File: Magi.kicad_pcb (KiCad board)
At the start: 6 copper layers, 122 x 84 mm, 366 parts, among them J1 Micro_SD_Card_Det2, J10 USB_C_Receptacle_USB2.0_16P, J11 USB_C_Receptacle_USB2.0_16P, J2 Bus_M.2_Socket_M, J3 Micro_SD_Card_Det2, J4 Bus_M.2_Socket_M, J5 Micro_SD_Card_Det2, J6 Bus_M.2_Socket_M, J7 RJ45_LED_Shielded, J8 Debug, J9 Magi Connector, Q1 DMN32D2LFB4, Q10 DMN32D2LFB4, Q11 DMN32D2LFB4, Q12 DMN32D2LFB4, Q13 DMN32D2LFB4, Q2 DMN32D2LFB4, Q3 DMN32D2LFB4, Q4 DMN32D2LFB4, Q5 DMN32D2LFB4, Q9 DMN32D2LFB4, T1 GA021G00, T2 GA021G00, T3 GA021G00, T4 GA021G00, U1 RT9742GGJ5, U10 DS1307Z+, U11 TPS56339DDC, U12 TPS56339DDC, U13 RTL8367N, U14 TPD4EUSB30, U15 TPD4EUSB30, U16 TPS259474A, U17 W25Q128JVS, U18 RP2040, U19 TVS2200DRV, U2 DS1307Z+, U20 ESD122DMYR, U21 ESD122DMYR, U22 TPD4EUSB30, U23 TPD4EUSB30, U24 TVS2200DRV, U25 TPS259470A, U26 TPS259474A, U27 TPS62933, U28 TPS259470A, U29 CYPD3177-24LQ, U3 TPS56339DDC, U30 TPS62933, U31 74LVC1G07, U32 74LVC1G07, U33 74LVC1G07, U4 TPS56339DDC, U5 RT9742GGJ5, U6 DS1307Z+, U7 TPS56339DDC, U8 TPS56339DDC, U9 RT9742GGJ5, Y1 32.768kHz, Y2 32.768kHz, Y3 32.768kHz, Y4 25MHz, Y5 ABM8-272-T3

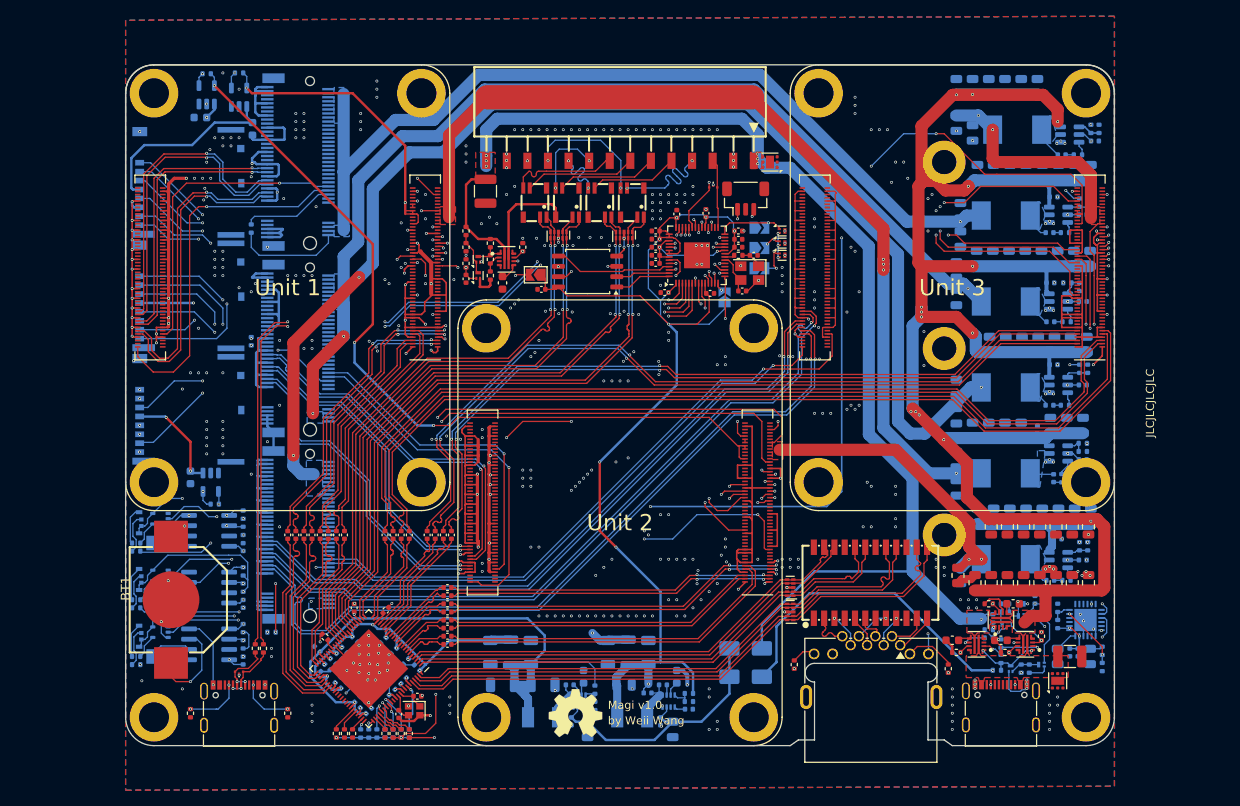
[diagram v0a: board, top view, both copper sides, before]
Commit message: Magi v2.0
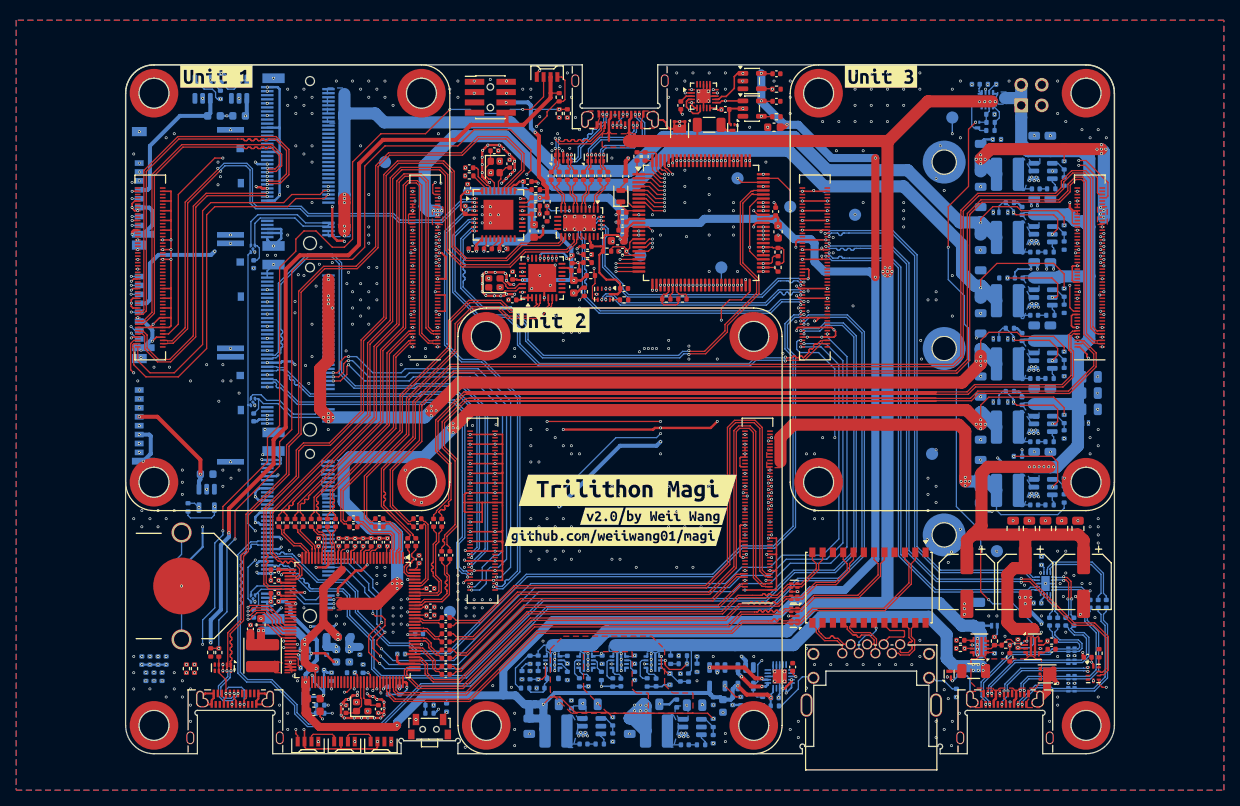
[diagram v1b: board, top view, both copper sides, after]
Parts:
- removed the C10 at (114.5, 109.5)
- removed the C11 at (204.5, 95.1)
- removed the C12 at (206.5, 95.1)
- removed the C13 at (208.5, 95.1)
- removed the C132 at (175.6, 72.5)
- removed the C137 at (164.4, 127.5)
- removed the C143 at (219.0, 123.0)
- removed the C2 at (120.0, 108.0)
- removed the C22 at (207.1, 63.3)
- removed the C68 at (135.0, 108.0)
- removed JP1, JP2, JP3: Unit PWR JP, Jumper:SolderJumper-2_P1.3mm_Open_TrianglePad1.0x1.5mm
- removed JP4: PWR JP, Jumper:SolderJumper-2_P1.3mm_Open_TrianglePad1.0x1.5mm
- removed JP5: POE JP, Jumper:SolderJumper-2_P1.3mm_Open_TrianglePad1.0x1.5mm
- removed Q10, Q11, Q12, Q13, Q5, Q9: DMN32D2LFB4, Package_DFN_QFN:Diodes_DFN1006-3
- removed the R1 at (101.3, 109.0)
- removed the R2 at (114.0, 51.0)
- removed the R3 at (114.5, 107.5)
- removed the R4 at (114.5, 105.5)
- removed the R69 at (211.5, 124.5)
- removed the R8 at (115.5, 70.2)
- removed SYM1: Magi v1.0, Magi:NAMEPLATE
- removed T1, T2, T3, T4: GA021G00, Magi:FILTER-SMD_6P-L4.5-W3.4_GA021G00
- removed the U1 at (114.0, 54.0)
- removed the U2 at (110.3, 107.5)
- removed Y5: ABM8-272-T3, Crystal:Crystal_SMD_3225-4Pin_3.2x2.5mm
- added C135: 6.8n, Capacitor_SMD:C_0402_1005Metric, B.Cu at (157.1, 126.2)
- added C144: 22u, Capacitor_SMD:C_0805_2012Metric, B.Cu at (170.2, 129.0)
- added C153: 22u, Capacitor_SMD:C_0805_2012Metric, F.Cu at (213.5, 107.2)
- added C185: 100n, Capacitor_SMD:C_0402_1005Metric, F.Cu at (156.5, 63.7)
- added C186: 100n, Capacitor_SMD:C_0402_1005Metric, F.Cu at (152.5, 63.7)
- added C187: 100n, Capacitor_SMD:C_0402_1005Metric, F.Cu at (153.5, 63.7)
- added C188: 100n, Capacitor_SMD:C_0402_1005Metric, F.Cu at (154.5, 63.7)
- added C189: 100n, Capacitor_SMD:C_0402_1005Metric, F.Cu at (155.5, 63.7)
- added C25: 100n, Capacitor_SMD:C_0402_1005Metric, B.Cu at (210.6, 83.6)
- added C26: 22u, Capacitor_SMD:C_0805_2012Metric, B.Cu at (212.1, 98.7)
- added C27: 22u, Capacitor_SMD:C_0805_2012Metric, B.Cu at (214.1, 98.7)
- added C28: 100n, Capacitor_SMD:C_0402_1005Metric, B.Cu at (210.2, 99.7)
- added C29: 100n, Capacitor_SMD:C_0402_1005Metric, B.Cu at (212.1, 88.7)
- added C30: 22u, Capacitor_SMD:C_0805_2012Metric, B.Cu at (205.5, 84.1)
- added C92: 100n, Capacitor_SMD:C_0402_1005Metric, B.Cu at (122.5, 127.5)
- added D10: WS2812B, Magi:LED-SMD_4P-L4.0-W1.7-R, F.Cu at (131.5, 133.5)
- added D11: 4.3v, Diode_SMD:D_SOD-523, B.Cu at (167.2, 125.8)
- added D12: 4.3v, Diode_SMD:D_SOD-523, B.Cu at (152.7, 125.7)
- added D13: RB161QS, Diode_SMD:D_SOD-882, B.Cu at (218.4, 94.2)
- added D14: RB161QS, Diode_SMD:D_SOD-882, B.Cu at (207.2, 119.2)
- added D15: RB161QS, Diode_SMD:D_SOD-882, B.Cu at (202.8, 125.0)
- added D6: RB161QS, Diode_SMD:D_SOD-882, B.Cu at (209.2, 91.6)
- added D7: WS2812B, Magi:LED-SMD_4P-L4.0-W1.7-R, F.Cu at (152.0, 51.5)
- added D8: WS2812B, Magi:LED-SMD_4P-L4.0-W1.7-R, F.Cu at (122.5, 133.5)
- added D9: WS2812B, Magi:LED-SMD_4P-L4.0-W1.7-R, F.Cu at (127.0, 133.5)
- added J12: USB_C_Receptacle, Magi:USB-C-SMD_TYPE-C-GT-USB-7007C, F.Cu at (161.0, 54.7)
- added L9: 5.6uH, Inductor_SMD:L_Changjiang_FTC404030S, B.Cu at (165.5, 132.2)
- added R10: 5.1k, Resistor_SMD:R_0402_1005Metric, F.Cu at (163.1, 61.3)
- added R100: 30R, Resistor_SMD:R_0402_1005Metric, B.Cu at (171.0, 133.9)
- added R101: 12k, Resistor_SMD:R_0402_1005Metric, B.Cu at (172.5, 133.2)
- added R102: 5.1k, Resistor_SMD:R_0402_1005Metric, B.Cu at (148.9, 125.3)
- added R103: 5.1k, Resistor_SMD:R_0402_1005Metric, B.Cu at (213.0, 111.2)
- added R104: 5.1k, Resistor_SMD:R_0402_1005Metric, B.Cu at (175.9, 128.5)
- added R105: 5.1k, Resistor_SMD:R_0402_1005Metric, B.Cu at (178.6, 128.5)
- added R106: 5.1k, Resistor_SMD:R_0402_1005Metric, F.Cu at (157.4, 76.0)
- added R107: 5.1k, Resistor_SMD:R_0402_1005Metric, F.Cu at (152.0, 68.8)
- added R108: 5.1k, Resistor_SMD:R_0402_1005Metric, F.Cu at (152.0, 66.9)
- added R109: 5.1k, Resistor_SMD:R_0402_1005Metric, F.Cu at (157.0, 74.4)
- added R11: 5.1k, Resistor_SMD:R_0402_1005Metric, F.Cu at (164.1, 61.3)
- added R110: 5.1k, Resistor_SMD:R_0402_1005Metric, F.Cu at (157.0, 73.4)
- added R111: 5.1k, Resistor_SMD:R_0402_1005Metric, F.Cu at (180.3, 53.0)
- added R112: 5.1k, Resistor_SMD:R_0402_1005Metric, F.Cu at (180.3, 56.4)
- added R113: 5.1k, Resistor_SMD:R_0402_1005Metric, B.Cu at (139.6, 129.3)
- added R114: 5.1k, Resistor_SMD:R_0402_1005Metric, F.Cu at (220.1, 122.6)
- added R115: 5.1k, Resistor_SMD:R_0402_1005Metric, F.Cu at (161.5, 79.0)
- added R5: 5.1k, Resistor_SMD:R_0402_1005Metric, B.Cu at (208.3, 76.3)
- added R66: 1.3k, Resistor_SMD:R_0402_1005Metric, F.Cu at (208.6, 121.6)
- added R7: 5.1k, Resistor_SMD:R_0402_1005Metric, B.Cu at (209.1, 67.0)
- added R74: 1k, Resistor_SMD:R_0402_1005Metric, B.Cu at (160.1, 126.2)
- added R9: 12k, Resistor_SMD:R_0402_1005Metric, B.Cu at (111.7, 53.7)
- added R92: 1.3k, Resistor_SMD:R_0402_1005Metric, B.Cu at (206.7, 57.1)
- added R93: 12k, Resistor_SMD:R_0402_1005Metric, B.Cu at (160.1, 133.0)
- added R94: 5.6k, Resistor_SMD:R_0402_1005Metric, B.Cu at (206.7, 56.1)
- added R95: 5.1k, Resistor_SMD:R_0402_1005Metric, B.Cu at (170.5, 124.4)
- added R97: 64.9k, Resistor_SMD:R_0402_1005Metric, B.Cu at (172.5, 131.2)
- added R98: 1.2k 0.5W, Resistor_SMD:R_1206_3216Metric, F.Cu at (172.0, 57.4)
- added R99: 100k, Resistor_SMD:R_0402_1005Metric, B.Cu at (149.9, 123.4)
- added SW1: SW_Push, Magi:SW-SMD_L4.7-W3.5-P3.35-EH, F.Cu at (137.5, 131.7)
- added TP1: TestPoint, TestPoint:TestPoint_Pad_D1.5mm, B.Cu at (190.0, 68.5)
- added TP10: TestPoint, TestPoint:TestPoint_Pad_D1.5mm, B.Cu at (218.9, 76.0)
- added TP11: TestPoint, TestPoint:TestPoint_Pad_D1.5mm, B.Cu at (207.5, 110.0)
- added TP12: TestPoint, TestPoint:TestPoint_Pad_D1.5mm, B.Cu at (132.0, 62.0)
- added TP13: TestPoint, TestPoint:TestPoint_Pad_D1.5mm, B.Cu at (140.0, 117.5)
- added TP2: TestPoint, TestPoint:TestPoint_Pad_D1.5mm, B.Cu at (199.5, 98.0)
- added TP3: TestPoint, TestPoint:TestPoint_Pad_D1.5mm, B.Cu at (202.0, 56.5)
- added TP4: TestPoint, TestPoint:TestPoint_Pad_D1.5mm, B.Cu at (163.5, 73.5)
- added TP5: TestPoint, TestPoint:TestPoint_Pad_D1.5mm, B.Cu at (175.5, 64.0)
- added TP6: TestPoint, TestPoint:TestPoint_Pad_D1.5mm, B.Cu at (182.0, 67.5)
- added TP7: TestPoint, TestPoint:TestPoint_Pad_D1.5mm, B.Cu at (173.5, 75.0)
- added TP8: TestPoint, TestPoint:TestPoint_Pad_D1.5mm, B.Cu at (175.2, 121.6)
- added TP9: TestPoint, TestPoint:TestPoint_Pad_D1.5mm, B.Cu at (158.2, 121.0)
- added U3: AP2151W, Package_TO_SOT_SMD:SOT-23-5, B.Cu at (109.5, 53.0)
- added U34: TPD4EUSB30, Package_SON:USON-10_2.5x1.0mm_P0.5mm, B.Cu at (216.7, 122.9)
- added U35: AP2151W, Package_TO_SOT_SMD:SOT-23-5, B.Cu at (173.0, 125.5)
- added U36: AP2151W, Package_TO_SOT_SMD:SOT-23-5, B.Cu at (176.5, 125.5)
- added U37: TS3USB221, Package_DFN_QFN:Texas_UQFN-10_1.5x2mm_P0.5mm, F.Cu at (159.0, 78.3)
- added U38: TPD6S300A, Package_DFN_QFN:WQFN-20-1EP_3x3mm_P0.4mm_EP1.7x1.7mm_ThermalVias, F.Cu at (171.3, 53.9)
- added U39: TVS2200DRV, Package_SON:WSON-6-1EP_2x2mm_P0.65mm_EP1x1.6mm, F.Cu at (168.3, 57.9)
- added U4: 74AUP1G125, Package_SON:Texas_X2SON-5_0.8x0.8mm_P0.48mm, B.Cu at (115.7, 72.7)
- added U40: HD3SS460, Magi:WQFN-28-1EP_3.5x5.5mm_P0.5mm_EP2.05x4.05mm_ThermalVias_SingleSided, F.Cu at (156.0, 69.5)
- added U41: TPD4EUSB30, Package_SON:USON-10_2.5x1.0mm_P0.5mm, F.Cu at (158.0, 61.5)
- added U42: AP2151W, Package_TO_SOT_SMD:SOT-23-5, F.Cu at (177.3, 52.0)
- added U43: TPD4EUSB30, Package_SON:USON-10_2.5x1.0mm_P0.5mm, F.Cu at (154.0, 61.5)
- added U44: AP2151W, Package_TO_SOT_SMD:SOT-23-5, F.Cu at (177.3, 55.4)
- added kibuzzard-69C4E3CF: G***, kibuzzard-69C4E3CF, B.Cu at (115.6, 69.0)
- added kibuzzard-69C4E40D: G***, kibuzzard-69C4E40D, B.Cu at (115.6, 83.0)
- added kibuzzard-69C4E42D: G***, kibuzzard-69C4E42D, B.Cu at (115.6, 97.0)
- added kibuzzard-69C50949: G***, kibuzzard-69C50949, F.Cu at (111.2, 51.4)
- added kibuzzard-69C5095C: G***, kibuzzard-69C5095C, F.Cu at (152.5, 81.5)
- added kibuzzard-69C50974: G***, kibuzzard-69C50974, F.Cu at (193.2, 51.4)
- added kibuzzard-69C50981: G***, kibuzzard-69C50981, B.Cu at (196.5, 52.4)
- added kibuzzard-69C5098A: G***, kibuzzard-69C5098A, B.Cu at (196.5, 75.4)
- added kibuzzard-69C509A0: G***, kibuzzard-69C509A0, B.Cu at (196.5, 98.4)
- added kibuzzard-6A5B14ED: G***, kibuzzard-6A5B14ED, F.Cu at (161.9, 102.5)
- added kibuzzard-6A5B154C: G***, kibuzzard-6A5B154C, F.Cu at (167.7, 105.7)
- added kibuzzard-6A5B1551: G***, kibuzzard-6A5B1551, F.Cu at (160.2, 108.2)
- added kibuzzard-6A5B157A: G***, kibuzzard-6A5B157A, F.Cu at (158.8, 105.7)
- BT1: value RTC Battery -> CR1220
- C100, C113: value 100u -> 100n; footprint Capacitor_SMD:C_1206_3216Metric -> Capacitor_SMD:C_0402_1005Metric; moved to F.Cu
- C101, C102, C104, C105, C106, C111, C114, C115, C154, C155, C162, C163, C40, C70, C78, C91, C93: moved to F.Cu
- C103, C108: value 100n -> 4.7u; footprint Capacitor_SMD:C_0402_1005Metric -> Capacitor_SMD:C_0603_1608Metric; moved to F.Cu
- C109: value 6p -> 100n
- C110: value 6p -> 4.7u; footprint Capacitor_SMD:C_0402_1005Metric -> Capacitor_SMD:C_0603_1608Metric
- C112, C99: value 100u -> 10u; footprint Capacitor_SMD:C_1206_3216Metric -> Capacitor_SMD:C_0603_1608Metric; moved to F.Cu
- C116: value 100n -> 1u; moved to F.Cu
- C117: value 1u -> 100n
- C118, C96: value 100n -> 1u
- C119, C127, C128: value 100n -> 18pf
- C120: value 1u -> 18pf
- C122: value 6.8n -> 100n; footprint Capacitor_SMD:C_0603_1608Metric -> Capacitor_SMD:C_0402_1005Metric
- C123: value 3.3u 100V -> 100n; footprint Capacitor_SMD:C_1210_3225Metric -> Capacitor_SMD:C_0402_1005Metric
- C124, C125: value 15p -> 100n
- C129, C32, C36, Q1, Q2: moved to B.Cu
- C13: renamed from C9; value 10u 25V -> 10u
- C130, C131: value 100n -> 6.8n; moved to B.Cu
- C132: renamed from C135; footprint Capacitor_SMD:C_0603_1608Metric -> Capacitor_SMD:C_0402_1005Metric
- C133: value 100n -> 10u 50V; footprint Capacitor_SMD:C_0402_1005Metric -> Capacitor_SMD:C_1210_3225Metric; moved to B.Cu
- C134: value 3.3u 100V -> 100n; footprint Capacitor_SMD:C_1210_3225Metric -> Capacitor_SMD:C_0402_1005Metric; moved to B.Cu
- C136: value 100n -> 6.8n
- C137: renamed from C144; footprint Capacitor_SMD:C_0603_1608Metric -> Capacitor_SMD:C_0402_1005Metric
- C138, C148: value 10u 50V -> 22u
- C139: value 100n 50V -> 100n
- C14, C145, C168, C169, C175, C176, C177, C178, C179, C181, C182, C183, C184, C51, C54, C71, C72, C76, C86: value 22u -> 100n; footprint Capacitor_SMD:C_0805_2012Metric -> Capacitor_SMD:C_0402_1005Metric
- C140: value 1u 50V -> 100n; footprint Capacitor_SMD:C_0805_2012Metric -> Capacitor_SMD:C_0402_1005Metric
- C141, C142, C147, C48: value 100n -> 22u; footprint Capacitor_SMD:C_0402_1005Metric -> Capacitor_SMD:C_0805_2012Metric
- C143: renamed from C153; footprint Capacitor_SMD:C_0603_1608Metric -> Capacitor_SMD:C_0402_1005Metric; moved to B.Cu
- C146: value 33n -> 100n; footprint Capacitor_SMD:C_0603_1608Metric -> Capacitor_SMD:C_0402_1005Metric
- C149: value 100n 50V -> 22u; footprint Capacitor_SMD:C_0402_1005Metric -> Capacitor_SMD:C_0805_2012Metric
- C150: value 100u -> 22u; footprint Capacitor_SMD:C_1206_3216Metric -> Capacitor_SMD:C_0805_2012Metric
- C151: value 100u -> 22u; footprint Capacitor_SMD:C_1206_3216Metric -> Capacitor_SMD:C_0805_2012Metric; moved to F.Cu
- C152: value 33n -> 22u; footprint Capacitor_SMD:C_0603_1608Metric -> Capacitor_SMD:C_0805_2012Metric; moved to F.Cu
- C157, C158, C159: value 22u -> 100u; footprint Capacitor_SMD:C_0805_2012Metric -> Capacitor_SMD:CP_Elec_6.3x5.7; moved to F.Cu
- C167: value 1u -> 100n; moved to B.Cu
- C170, C172, C173, C174, C50: value 22u -> 100n; footprint Capacitor_SMD:C_0805_2012Metric -> Capacitor_SMD:C_0402_1005Metric; moved to B.Cu
- C171: value 22u -> 10u; footprint Capacitor_SMD:C_0805_2012Metric -> Capacitor_SMD:C_0603_1608Metric; moved to B.Cu
- C180, C79: value 22u -> 10u; footprint Capacitor_SMD:C_0805_2012Metric -> Capacitor_SMD:C_0603_1608Metric
- C21, C41, C42, C43, C44, C59, C60, C75, C81, C82, C83, C84, C85, C89, C90: value 22u -> 100n; footprint Capacitor_SMD:C_0805_2012Metric -> Capacitor_SMD:C_0402_1005Metric; moved to F.Cu
- C31, C33, C34: value 100n -> 22u; footprint Capacitor_SMD:C_0402_1005Metric -> Capacitor_SMD:C_0805_2012Metric; moved to B.Cu
- C35: value 100n -> 10u; footprint Capacitor_SMD:C_0402_1005Metric -> Capacitor_SMD:C_0603_1608Metric; moved to B.Cu
- C39, C69: value 10u 25V -> 100n; footprint Capacitor_SMD:C_0603_1608Metric -> Capacitor_SMD:C_0402_1005Metric; moved to F.Cu
- C57, C95: value 100n -> 10u; footprint Capacitor_SMD:C_0402_1005Metric -> Capacitor_SMD:C_0603_1608Metric
- C73, C74: value 22u -> 18pf; footprint Capacitor_SMD:C_0805_2012Metric -> Capacitor_SMD:C_0402_1005Metric; moved to F.Cu
- C80: value 22u -> 1u; footprint Capacitor_SMD:C_0805_2012Metric -> Capacitor_SMD:C_0402_1005Metric
- C97, C98: value 100n -> 10u; footprint Capacitor_SMD:C_0402_1005Metric -> Capacitor_SMD:C_0603_1608Metric; moved to F.Cu
- D1, D2, D3: value LED_Dual_AAKK -> RB161QS; footprint Magi:LED-ARRAY-SMD_4P-L3.0-W1.5-L-FD -> Diode_SMD:D_SOD-882
- D4, D5: value M7 -> RB161QS; footprint Diode_SMD:D_SMA -> Diode_SMD:D_SOD-882
- FB1, FB2: value FerriteBead -> 220R; footprint Inductor_SMD:L_1206_3216Metric -> Inductor_SMD:L_0603_1608Metric
- J1, J3, J5: footprint Magi:TF-SMD_503398-1892 -> Magi:SDCARD_MOLEX_503398-1892
- J10: value USB_C_Receptacle_USB2.0_16P -> Conn_02x02_Odd_Even; footprint Magi:USB-C-SMD_TYPEC-304J-BCP16 -> Connector_PinHeader_2.54mm:PinHeader_2x02_P2.54mm_Vertical; moved to B.Cu
- J11: value USB_C_Receptacle_USB2.0_16P -> USB_C_Receptacle; footprint Magi:USB-C-SMD_TYPEC-304J-BCP16 -> Magi:USB-C-SMD_TYPE-C-GT-USB-7007C
- J7: footprint Magi:RJ45-TH_MJ88B-B011-RVL11-P -> Magi:RJ45-TH_RJ45-005-202-11
- J8: value Debug -> USB_C_Receptacle; footprint Connector_JST:JST_SH_BM03B-SRSS-TB_1x03-1MP_P1.00mm_Vertical -> Magi:USB-C-SMD_TYPE-C-GT-USB-7007C
- J9: value Magi Connector -> Conn_02x04; footprint Magi:HDR-SMD_14P-P2.54-H-F-L11.5 -> Magi:PinHeader_2x04_P1.27mm_Vertical_SMD_MountingPegs
- L1, L2: footprint Inductor_SMD:L_Sunlord_MWSA0603S -> Inductor_SMD:L_Changjiang_FTC404030S
- L3, L5: value 5.6uH -> 4.7uH; footprint Inductor_SMD:L_Sunlord_MWSA0603S -> Inductor_SMD:L_Changjiang_FTC404030S
- L4, L6: value 4.7uH -> 5.6uH; footprint Inductor_SMD:L_Sunlord_MWSA0603S -> Inductor_SMD:L_Changjiang_FTC404030S
- L7: value 2.2u 4.5A -> 2.2uH; footprint Inductor_SMD:L_Sunlord_MWSA0402S -> Inductor_SMD:L_Changjiang_FTC404030S; moved to F.Cu
- L8: value 2.2u 4.5A -> 4.7uH; footprint Inductor_SMD:L_Sunlord_MWSA0402S -> Inductor_SMD:L_Changjiang_FTC404030S
- Module1, Module2, Module3: value ComputeModule4-CM4 -> Compute Module
- R1: renamed from R5; value 52.3k 1% -> 64.9k
- R12, R23, R88: value 1k -> 37.4k
- R13, R24: value 12k 1% -> 64.9k
- R14, R15, R25, R26: value 4.7k -> 30R
- R16, R27: value 52.3k 1% -> 5.1k
- R17, R28: value 30 1% -> 12k
- R18, R29: value 10k 1% -> 5.1k
- R19, R30: value 10k -> 12k
- R2: renamed from R9; value 30.9k 1% -> 37.4k
- R20, R31: value 30.9k 1% -> 12k
- R21, R32: value 30 1% -> 5.1k; moved to F.Cu
- R22, R33: value 10k 1% -> 5.1k; moved to F.Cu
- R3: renamed from R6; value 30 1% -> 30R
- R34: value 2.49K -> 5.1k; moved to B.Cu
- R35, R38: value 4.7k -> 5.1k
- R36, R39, R40: value 4.7k -> 5.1k; moved to B.Cu
- R37: value 4.7k -> 2.49K
- R4: renamed from R10; value 30 1% -> 30R
- R41, R42, R43: value 4.7k -> 1k; moved to B.Cu
- R44, R45, R47, R48, R49, R50: value 4.7k -> 1k
- R46: value 470R -> 1k; moved to B.Cu
- R51: value 470R -> 100k
- R52: value 4.7k -> 100k; moved to F.Cu
- R53: value 100k -> 5.1k
- R54: value 220k 1% -> 5.1k
- R55, R82: value 20k -> 5.1k
- R56: value 2.74k 1% -> 12k
- R57: value 12.7k 1% -> 5.1k
- R58: value 27.4 -> 5.1k
- R59: value 27.4 -> 100k
- R6: renamed from R7; value 10k 1% -> 12k
- R60: value 4.7k -> 100k
- R61: value 1k -> 5.1k
- R63: value 5.1k -> 2.49K
- R64: value 220k 1% -> 100k; moved to F.Cu
- R65: value 220k 1% -> 100k; moved to B.Cu
- R67: value 220k 1% -> 5.6k
- R68, R80: value 100k -> 1.3k
- R69: renamed from R66; value 100k -> 12k
- R70: value 2.26k 1% -> 5.1k
- R71: value 953 -> 5.1k; moved to B.Cu
- R72: value 13k 1% -> 5.6k; moved to F.Cu
- R73: value 30.9k 1% -> 100k
- R75, R85: value 10k 1% -> 1k
- R76: value 15k -> 1k; footprint Capacitor_SMD:C_0402_1005Metric -> Resistor_SMD:R_0402_1005Metric; moved to F.Cu
- R77: value 220k 1% -> 100k
- R79: value 2.74k 1% -> 5.6k
- R8: renamed from R11; value 10k 1% -> 12k
- R81: value 2.4k -> 5.1k
- R83: value 12.7k 1% -> 100k
- R84: value 3.74k 1% -> 1k
- R86: renamed from R74; value 953 -> 1k
- R87, R91: value 1k -> 100k
- R89: value 1k -> 30R
- R90: value 5.1k -> 1.2k 0.5W; footprint Resistor_SMD:R_0402_1005Metric -> Resistor_SMD:R_1206_3216Metric; moved to F.Cu
- R96: renamed from R86; value 1.2k 1% -> 1k; moved to B.Cu
- TR1: value H2456G -> H2449G; footprint Magi:XFMR-SMD-24_L16.6-W9.0-LS9.6-BL -> Magi:RJ45-SMD_24P_L15.6-W8.7_H24308C
- U10, U6: value DS1307Z+ -> TPS56339DDC; footprint Package_SO:SOIC-8_3.9x4.9mm_P1.27mm -> Package_TO_SOT_SMD:SOT-23-6
- U11, U7: value TPS56339DDC -> AP2151W; footprint Package_TO_SOT_SMD:SOT-23-6 -> Package_TO_SOT_SMD:SOT-23-5
- U12, U8: value TPS56339DDC -> 74AUP1G125; footprint Package_TO_SOT_SMD:SOT-23-6 -> Package_SON:Texas_X2SON-5_0.8x0.8mm_P0.48mm
- U13: value RTL8367N -> RTL8367S-CG; footprint Magi:QFN-88_EP_10x10_Pitch0.4mm2 -> Package_QFP:LQFP-128_14x14mm_P0.4mm
- U14, U15: footprint Magi:USON-10_2.5x1.0mm_P0.5mm -> Package_SON:USON-10_2.5x1.0mm_P0.5mm
- U16: value TPS259474A -> USB2514B; footprint Magi:RPW0010A-MFG -> Package_DFN_QFN:QFN-36-1EP_6x6mm_P0.5mm_EP3.7x3.7mm
- U17: value W25Q128JVS -> CH390H; footprint Package_SO:SOIC-8_5.23x5.23mm_P1.27mm -> Package_DFN_QFN:QFN-32-1EP_5x5mm_P0.5mm_EP3.45x3.45mm
- U18: value RP2040 -> STM32G0B1VETx; footprint Package_DFN_QFN:QFN-56-1EP_7x7mm_P0.4mm_EP3.2x3.2mm -> Package_QFP:LQFP-100_14x14mm_P0.5mm
- U19: value TVS2200DRV -> TPD4EUSB30; footprint Package_SON:WSON-6-1EP_2x2mm_P0.65mm_EP1x1.6mm -> Package_SON:USON-10_2.5x1.0mm_P0.5mm
- U20, U21: value ESD122DMYR -> TPS259470A; footprint Magi:DMY0003A -> Magi:RPW0010A-MFG; moved to B.Cu
- U22: value TPD4EUSB30 -> TPS259470A; footprint Magi:USON-10_2.5x1.0mm_P0.5mm -> Magi:RPW0010A-MFG
- U23: value TPD4EUSB30 -> TPS259470A; footprint Magi:USON-10_2.5x1.0mm_P0.5mm -> Magi:RPW0010A-MFG; moved to B.Cu
- U24: value TVS2200DRV -> TPS259470A; footprint Package_SON:WSON-6-1EP_2x2mm_P0.65mm_EP1x1.6mm -> Magi:RPW0010A-MFG; moved to B.Cu
- U26: value TPS259474A -> TPS56339DDC; footprint Magi:RPW0010A-MFG -> Package_TO_SOT_SMD:SOT-23-6; moved to B.Cu
- U27: value TPS62933 -> TPS259470A; footprint Package_TO_SOT_SMD:SOT-583-8 -> Magi:RPW0010A-MFG
- U28: value TPS259470A -> TPS56339DDC; footprint Magi:RPW0010A-MFG -> Package_TO_SOT_SMD:SOT-23-6; moved to B.Cu
- U29: value CYPD3177-24LQ -> TVS2200DRV; footprint Package_DFN_QFN:QFN-24-1EP_4x4mm_P0.5mm_EP2.75x2.75mm -> Package_SON:WSON-6-1EP_2x2mm_P0.65mm_EP1x1.6mm; moved to F.Cu
- U30: value TPS62933 -> TPD6S300A; footprint Package_TO_SOT_SMD:SOT-583-8 -> Package_DFN_QFN:WQFN-20-1EP_3x3mm_P0.4mm_EP1.7x1.7mm_ThermalVias
- U31: value 74LVC1G07 -> FUSB340TMX; footprint Package_TO_SOT_SMD:SOT-353_SC-70-5 -> Magi:QFN-18-1EP_2x2.8mm_P0.4mm_EP1.05x1.85mm
- U32: value 74LVC1G07 -> TPD4EUSB30; footprint Package_TO_SOT_SMD:SOT-353_SC-70-5 -> Package_SON:USON-10_2.5x1.0mm_P0.5mm
- U33: value 74LVC1G07 -> TS3USB221; footprint Package_TO_SOT_SMD:SOT-353_SC-70-5 -> Package_DFN_QFN:Texas_UQFN-10_1.5x2mm_P0.5mm; moved to F.Cu
- U5, U9: value RT9742GGJ5 -> TPS56339DDC; footprint Package_TO_SOT_SMD:TSOT-23-5 -> Package_TO_SOT_SMD:SOT-23-6
- Y1, Y2: value 32.768kHz -> 25MHz; footprint Crystal:Crystal_SMD_3215-2Pin_3.2x1.5mm -> Crystal:Crystal_SMD_2016-4Pin_2.0x1.6mm; moved to F.Cu
- Y3: value 32.768kHz -> 24MHz; footprint Crystal:Crystal_SMD_3215-2Pin_3.2x1.5mm -> Crystal:Crystal_SMD_2016-4Pin_2.0x1.6mm; moved to F.Cu
- Y4: value 25MHz -> 32.768kHz; footprint Crystal:Crystal_SMD_2016-4Pin_2.0x1.6mm -> Crystal:Crystal_SMD_2012-2Pin_2.0x1.2mm
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- renumbered C15 to C1, C28 to C10, C29 to C11, C30 to C12, C5 to C15, C7 to C16, C1 to C17, C3 to C18, C6 to C19, C16 to C2, C8 to C20, C4 to C22, C17 to C3, C25 to C4, C26 to C5, C27 to C6, C92 to C68, C18 to C7, C19 to C8, C20 to C9, U3 to U1, U4 to U2
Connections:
- net /Unit 1A/BUCK_SW renamed /Unit 1/BUCK_SW_5
- net /Unit 1A/CM_5V renamed /Unit 1/CM_5V
- net /Unit 1A/ETH_P0_N renamed /Unit 1/ETH_P0-
- net /Unit 1A/ETH_P0_P renamed /Unit 1/ETH_P0+
- net /Unit 1A/ETH_P1_N renamed /Unit 1/ETH_P1-
- net /Unit 1A/ETH_P1_P renamed /Unit 1/ETH_P1+
- net /Unit 1A/ETH_P3_N renamed /Unit 1/ETH_P3-
- net /Unit 1A/SD_CLK renamed /Unit 1/SD_CLK
- net /Unit 1A/SD_CMD renamed /Unit 1/SD_CMD
- net /Unit 1A/SD_DAT0 renamed /Unit 1/SD_DAT0
- net /Unit 1A/SD_DAT1 renamed /Unit 1/SD_DAT1
- net /Unit 1A/SD_DAT2 renamed /Unit 1/SD_DAT2
- net /Unit 1A/SD_DAT3 renamed /Unit 1/SD_DAT3
- net /Unit 1A/SD_PWR renamed /Unit 1/SD_PWR
- net /Unit 1B/BUCK_SW renamed /Unit 1/BUCK_SW_3
- net /Unit 1B/PCIE_CLK_N renamed /Unit 1/PCIE_CLK-
- net /Unit 1B/PCIE_CLK_P renamed /Unit 1/PCIE_CLK+
- net /Unit 1B/PCIE_CLK_nREQ renamed /Unit 1/PCIE_CLK_nREQ
- net /Unit 1B/PCIE_nRST renamed /Unit 1/PCIE_nRST
- net /Unit 2A/SD_CLK renamed /Unit 2/SD_CLK
- net /Unit 2A/SD_CMD renamed /Unit 2/SD_CMD
- net /Unit 2A/SD_DAT0 renamed /Unit 2/SD_DAT0
- net /Unit 2A/SD_DAT1 renamed /Unit 2/SD_DAT1
- net /Unit 2A/SD_DAT2 renamed /Unit 2/SD_DAT2
- net /Unit 2A/SD_DAT3 renamed /Unit 2/SD_DAT3
- net /Unit 2B/PCIE_CLK_N renamed /Unit 2/PCIE_CLK-
- net /Unit 2B/PCIE_CLK_P renamed /Unit 2/PCIE_CLK+
- net /Unit 2B/PCIE_CLK_nREQ renamed /Unit 2/PCIE_CLK_nREQ
- net /Unit 2B/PCIE_RX_N renamed /Unit 2/PCIE_RX-
- net /Unit 2B/PCIE_RX_P renamed /Unit 2/PCIE_RX+
- net /Unit 2B/PCIE_nRST renamed /Unit 2/PCIE_nRST
- net /Unit 3A/ETH_P1_P renamed /Unit 3/ETH_P1+
- net /Unit 3A/SD_CLK renamed /Unit 3/SD_CLK
- net /Unit 3A/SD_CMD renamed /Unit 3/SD_CMD
- net /Unit 3A/SD_DAT0 renamed /Unit 3/SD_DAT0
- net /Unit 3A/SD_DAT1 renamed /Unit 3/SD_DAT1
- net /Unit 3A/SD_DAT2 renamed /Unit 3/SD_DAT2
- net /Unit 3A/SD_DAT3 renamed /Unit 3/SD_DAT3
- net /Unit 3B/PCIE_CLK_N renamed /Unit 3/PCIE_CLK-
- net /Unit 3B/PCIE_CLK_P renamed /Unit 3/PCIE_CLK+
- net /Unit 3B/PCIE_CLK_nREQ renamed /Unit 3/PCIE_CLK_nREQ
- net /Unit 3B/PCIE_RX_N renamed /Unit 3/PCIE_RX-
- net /Unit 3B/PCIE_RX_P renamed /Unit 3/PCIE_RX+
- net /Unit 3B/PCIE_nRST renamed /Unit 3/PCIE_nRST
- net U1_RUN_PG renamed /Controller/PE4
- net U1_UART0_RX renamed /Controller/PC10_USART4_TX
- net U1_UART0_TX renamed /Controller/PC11_USART4_RX
- BT1 pad 1: +BATT -> Net-(BT1-+)
- BT1 pad 2: GND -> Net-(BT1--)
- C100 pad 1: /Ethernet Switch/ANALOG_3V3 -> /Ethernet Switch/1V1
- C101 pad 1: /Ethernet Switch/ANALOG_1V1 -> GND
- C101 pad 2: GND -> +3V3
- C102 pad 1: /Ethernet Switch/ANALOG_1V1 -> GND
- C102 pad 2: GND -> +3V3
- C103 pad 1: /Ethernet Switch/ANALOG_1V1 -> +3V3
- C104 pad 1: /Ethernet Switch/ANALOG_1V1 -> GND
- C104 pad 2: GND -> +3V3
- C105 pad 1: /Ethernet Switch/ANALOG_1V1 -> GND
- C105 pad 2: GND -> +3V3
- C106 pad 1: /Ethernet Switch/ANALOG_1V1 -> GND
- C106 pad 2: GND -> +3V3
- C107 pad 1: /Ethernet Switch/ANALOG_1V1 -> GND
- C107 pad 2: GND -> +3V3
- C108 pad 1: /Ethernet Switch/ANALOG_1V1 -> +3V3
- C109 pad 1: Net-(U13-XTALO) -> GND
- C109 pad 2: GND -> +3V3
- C11 pad 1: /Unit 1B/M2_3V3 -> /Unit 1/M2_3V3
- C110 pad 1: Net-(U13-XTALI) -> +3V3
- C111 pad 1: AUX_3V3 -> GND
- C111 pad 2: GND -> +3V3
- C112 pad 1: AUX_1V1 -> +3V3
- C113 pad 1: /Ethernet Switch/ANALOG_1V1 -> GND
- C113 pad 2: GND -> +3V3
- C114 pad 1: AUX_1V1 -> GND
- C114 pad 2: GND -> +3V3
- C115 pad 1: AUX_1V1 -> GND
- C115 pad 2: GND -> +3V3
- C116 pad 1: AUX_1V1 -> GND
- C116 pad 2: GND -> Net-(U18-VREF+)
- C117 pad 2: Net-(U18-VREG_VOUT) -> /Controller/~{MCU_RST}
- C118 pad 2: Net-(U18-VREG_VOUT) -> Net-(U17-RSVD)
- C119 pad 2: Net-(U18-VREG_VOUT) -> Net-(U16-XTALIN/CLKIN)
- C12 pad 1: /Unit 1B/M2_3V3 -> /Unit 1/M2_3V3
- C120 pad 2: AUX_3V3 -> Net-(U16-XTALOUT)
- C121 pad 1: AUX_3V3 -> Net-(U16-PLLFILT)
- C122 pad 1: Net-(U16-dVdt) -> Net-(U16-CRFILT)
- C123 pad 1: GND -> /Controller/MDIT-
- C123 pad 2: CONN_VBUS -> /Controller/ETH_P0+
- C124 pad 1: GND -> /Controller/MDIT+
- C124 pad 2: Net-(U18-XIN) -> /Controller/ETH_P0-
- C125 pad 1: GND -> /Controller/MDIR-
- C125 pad 2: Net-(C125-Pad2) -> /Controller/ETH_P1+
- C126 pad 1: AUX_3V3 -> /Controller/MDIR+
- C126 pad 2: GND -> /Controller/ETH_P1-
- C127 pad 1: AUX_3V3 -> GND
- C127 pad 2: GND -> Net-(U18-PC14)
- C128 pad 1: AUX_3V3 -> GND
- C128 pad 2: GND -> Net-(U18-PC15)
- C129 pad 1: AUX_3V3 -> Net-(D11-K)
- C130 pad 1: AUX_3V3 -> Net-(U20-dVdt)
- C131 pad 1: AUX_3V3 -> Net-(U21-dVdt)
- C132 pad 1: Net-(U25-dVdt) -> Net-(U22-dVdt)
- C133 pad 1: AUX_3V3 -> VCON
- C134 pad 1: GND -> Net-(D12-K)
- C134 pad 2: /Power/VBUS -> GND
- C136 pad 1: Net-(U27-SW) -> Net-(U24-dVdt)
- C136 pad 2: Net-(U27-BST) -> GND
- C137 pad 1: Net-(U26-dVdt) -> Net-(U25-dVdt)
- C138 pad 1: /Power/PWR_MUX -> GND
- C138 pad 2: GND -> /Power/PWR_MUX
- C139 pad 1: /Power/PWR_MUX -> GND
- C139 pad 2: GND -> /Power/PWR_MUX
- C14 pad 2: +20V -> /Unit 1/M2_3V3
- C140 pad 1: GND -> /Power/BUCK_SW_3
- C140 pad 2: Net-(U29-VCCD) -> Net-(C140-Pad2)
- C141 pad 1: GND -> +3V3
- C141 pad 2: /Power/CYPD3177_VDDD -> GND
- C142 pad 1: GND -> +3V3
- C142 pad 2: /Power/CYPD3177_VDDD -> GND
- C143 pad 1: Net-(U28-dVdt) -> Net-(U27-dVdt)
- C145 pad 1: AUX_3V3 -> GND
- C145 pad 2: GND -> /Power/PWR_MUX
- C146 pad 1: Net-(U27-SS) -> /Power/BUCK_SW_5
- C146 pad 2: GND -> Net-(C146-Pad2)
- C147 pad 1: Net-(U30-SW) -> +5V
- C147 pad 2: Net-(U30-BST) -> GND
- C148 pad 1: /Power/PWR_MUX -> +5V
- C149 pad 1: /Power/PWR_MUX -> +20V
- C15 pad 1: U1_ETH_P0_N -> /Ethernet Switch/P4MDIB-
- C150 pad 1: AUX_1V1 -> +20V
- C151 pad 1: AUX_1V1 -> +20V
- C152 pad 1: Net-(U30-SS) -> +20V
- C16 pad 1: U1_ETH_P0_P -> /Ethernet Switch/P4MDIB+
- C160 pad 1: UNIT1_CM_EN -> +3V3
- C161 pad 1: UNIT1_CM_EN -> +3V3
- C162 pad 1: UNIT2_CM_EN -> Net-(U30-VBIAS)
- C163 pad 1: UNIT2_CM_EN -> +3V3
- C164 pad 1: UNIT3_CM_EN -> /USB/USB_PORT_SS_RX1-
- C164 pad 2: GND -> /USB/USB_MUX_SS_RX1-
- C165 pad 1: UNIT3_CM_EN -> /USB/USB_PORT_SS_RX1+
- C165 pad 2: GND -> /USB/USB_MUX_SS_RX1+
- C166 pad 1: PWR_EN -> /USB/USB_PORT_SS_RX2-
- C166 pad 2: GND -> /USB/USB_MUX_SS_RX2-
- C167 pad 1: /Control/POE_EN -> /USB/USB_PORT_SS_RX2+
- C167 pad 2: GND -> /USB/USB_MUX_SS_RX2+
- C168 pad 1: +20V -> /USB/USB_PORT_SS_TX1-
- C168 pad 2: GND -> /USB/USB_MUX_SS_TX1-
- C169 pad 1: +20V -> /USB/USB_PORT_SS_TX1+
- C169 pad 2: GND -> /USB/USB_MUX_SS_TX1+
- C17 pad 1: U1_ETH_P1_P -> /Ethernet Switch/P4MDIA+
- C170 pad 1: +20V -> /USB/USB_PORT_SS_TX2-
- C170 pad 2: GND -> /USB/USB_MUX_SS_TX2-
- C171 pad 1: +20V -> +3V3
- C172 pad 1: +20V -> /USB/USB_PORT_SS_TX2+
- C172 pad 2: GND -> /USB/USB_MUX_SS_TX2+
- C173 pad 1: +20V -> +3V3
- C174 pad 1: +20V -> +3V3
- C175 pad 1: +20V -> +3V3
- C176 pad 1: +20V -> +3V3
- C177 pad 1: +20V -> +3V3
- C178 pad 1: +20V -> Net-(U38-VBIAS)
- C179 pad 1: +20V -> +3V3
- C18 pad 1: U1_ETH_P1_N -> /Ethernet Switch/P4MDIA-
- C180 pad 1: +20V -> +3V3
- C181 pad 1: +20V -> +3V3
- C182 pad 1: +20V -> /Interconnect/USB_PORT_RX1+
- C182 pad 2: GND -> /Interconnect/USB_RX1+
- C183 pad 1: +20V -> /Interconnect/USB_PORT_RX1-
- C183 pad 2: GND -> /Interconnect/USB_RX1-
- C184 pad 1: +20V -> /Interconnect/USB_PORT_TX1+
- C184 pad 2: GND -> /Interconnect/USB_TX1+
- C19 pad 1: U1_ETH_P2_N -> /Ethernet Switch/P4MDID-
- C19 pad 2: /Unit 1A/ETH_P2_N -> /Unit 1/ETH_P2-
- C20 pad 1: U1_ETH_P2_P -> /Ethernet Switch/P4MDID+
- C20 pad 2: /Unit 1A/ETH_P2_P -> /Unit 1/ETH_P2+
- C21 pad 1: GND -> /Ethernet Switch/P4MDIC-
- C21 pad 2: +20V -> /Unit 1/ETH_P3+
- C22 pad 1: U1_ETH_P3_N -> /Ethernet Switch/P4MDIC+
- C31 pad 1: U2_ETH_P1_P -> /Unit 2/M2_3V3
- C31 pad 2: /Unit 2A/ETH_P1_P -> GND
- C32 pad 1: U2_ETH_P3_P -> /Unit 2/BUCK_SW_5
- C32 pad 2: /Unit 2A/ETH_P3_P -> Net-(C32-Pad2)
- C33 pad 1: U2_ETH_P1_N -> /Unit 2/CM_5V
- C33 pad 2: /Unit 2A/ETH_P1_N -> GND
- C34 pad 1: U2_ETH_P3_N -> /Unit 2/CM_5V
- C34 pad 2: /Unit 2A/ETH_P3_N -> GND
- C35 pad 1: U2_ETH_P0_N -> /Unit 2/SD_PWR
- C35 pad 2: /Unit 2A/ETH_P0_N -> GND
- C36 pad 1: U2_ETH_P2_N -> GND
- C36 pad 2: /Unit 2A/ETH_P2_N -> /Unit 2/M2_3V3
- C37 pad 1: U2_ETH_P0_P -> /Ethernet Switch/P1MDIB-
- C37 pad 2: /Unit 2A/ETH_P0_P -> /Unit 2/ETH_P0-
- C38 pad 1: U2_ETH_P2_P -> /Ethernet Switch/P1MDIB+
- C38 pad 2: /Unit 2A/ETH_P2_P -> /Unit 2/ETH_P0+
- C39 pad 1: /Unit 2A/SD_PWR -> /Ethernet Switch/P1MDIA+
- C39 pad 2: GND -> /Unit 2/ETH_P1+
- C40 pad 1: GND -> /Ethernet Switch/P1MDIA-
- C40 pad 2: /Unit 2A/CM_5V -> /Unit 2/ETH_P1-
- C41 pad 1: GND -> /Ethernet Switch/P1MDID-
- C41 pad 2: +20V -> /Unit 2/ETH_P2-
- C42 pad 1: GND -> /Ethernet Switch/P1MDID+
- C42 pad 2: +20V -> /Unit 2/ETH_P2+
- C43 pad 1: GND -> /Ethernet Switch/P1MDIC-
- C43 pad 2: +20V -> /Unit 2/ETH_P3+
- C44 pad 1: GND -> /Ethernet Switch/P1MDIC+
- C44 pad 2: +20V -> /Unit 2/ETH_P3-
- C48 pad 1: /Unit 2A/BUCK_SW -> GND
- C48 pad 2: Net-(C48-Pad2) -> +20V
- C49 pad 1: /Unit 2A/CM_5V -> GND
- C49 pad 2: GND -> +20V
- C50 pad 1: /Unit 2A/CM_5V -> GND
- C50 pad 2: GND -> +20V
- C51 pad 1: GND -> /Unit 3/BUCK_SW_3
- C51 pad 2: +20V -> Net-(C51-Pad2)
- C52 pad 1: GND -> /Unit 3/M2_3V3
- C52 pad 2: +20V -> GND
- C53 pad 1: GND -> /Unit 3/M2_3V3
- C53 pad 2: +20V -> GND
- C54 pad 1: GND -> /Unit 3/BUCK_SW_5
- C54 pad 2: +20V -> Net-(C54-Pad2)
- C55 pad 1: GND -> /Unit 3/CM_5V
- C55 pad 2: +20V -> GND
- C56 pad 1: GND -> /Unit 3/CM_5V
- C56 pad 2: +20V -> GND
- C57 pad 1: GND -> /Unit 3/SD_PWR
- C57 pad 2: +20V -> GND
- C58 pad 1: /Unit 2B/BUCK_SW -> GND
- C58 pad 2: Net-(C58-Pad2) -> /Unit 3/M2_3V3
- C59 pad 1: /Unit 2B/M2_3V3 -> /Ethernet Switch/P2MDIB-
- C59 pad 2: GND -> /Unit 3/ETH_P0-
- C60 pad 1: /Unit 2B/M2_3V3 -> /Ethernet Switch/P2MDIB+
- C60 pad 2: GND -> /Unit 3/ETH_P0+
- C61 pad 1: U3_ETH_P1_P -> /Ethernet Switch/P2MDIA-
- C62 pad 1: U3_ETH_P3_P -> /Ethernet Switch/P2MDIA+
- C62 pad 2: /Unit 3A/ETH_P3_P -> /Unit 3/ETH_P1-
- C63 pad 1: U3_ETH_P1_N -> /Ethernet Switch/P2MDID+
- C63 pad 2: /Unit 3A/ETH_P1_N -> /Unit 3/ETH_P2-
- C64 pad 1: U3_ETH_P3_N -> /Ethernet Switch/P2MDID-
- C64 pad 2: /Unit 3A/ETH_P3_N -> /Unit 3/ETH_P2+
- C65 pad 1: U3_ETH_P0_N -> /Ethernet Switch/P2MDIC-
- C65 pad 2: /Unit 3A/ETH_P0_N -> /Unit 3/ETH_P3+
- C66 pad 1: U3_ETH_P2_N -> /Ethernet Switch/P2MDIC+
- C66 pad 2: /Unit 3A/ETH_P2_N -> /Unit 3/ETH_P3-
- C67 pad 1: U3_ETH_P0_P -> /Ethernet Switch/ANALOG_1V1
- C67 pad 2: /Unit 3A/ETH_P0_P -> GND
- C68 pad 1: /Ethernet Switch/ANALOG_3V3 -> /Ethernet Switch/ANALOG_1V1
- C69 pad 1: /Unit 3A/SD_PWR -> /Ethernet Switch/ANALOG_1V1
- C70 pad 1: GND -> /Ethernet Switch/ANALOG_1V1
- C70 pad 2: /Unit 3A/CM_5V -> GND
- C71 pad 1: GND -> /Ethernet Switch/ANALOG_1V1
- C71 pad 2: +20V -> GND
- C72 pad 1: GND -> /Ethernet Switch/ANALOG_1V1
- C72 pad 2: +20V -> GND
- C73 pad 2: +20V -> Net-(U13C-XTALI)
- C74 pad 2: +20V -> Net-(U13C-XTALO)
- C75 pad 1: GND -> /Ethernet Switch/1V1
- C75 pad 2: +20V -> GND
- C76 pad 1: GND -> /Ethernet Switch/1V1
- C76 pad 2: +20V -> GND
- C77 pad 1: GND -> /Ethernet Switch/1V1
- C77 pad 2: +20V -> GND
- C78 pad 1: /Unit 3A/BUCK_SW -> /Ethernet Switch/ANALOG_1V1
- C78 pad 2: Net-(C78-Pad2) -> GND
- C79 pad 1: /Unit 3A/CM_5V -> /Ethernet Switch/ANALOG_3V3
- C80 pad 1: /Unit 3A/CM_5V -> /Ethernet Switch/ANALOG_3V3
- C81 pad 1: GND -> /Ethernet Switch/ANALOG_1V1
- C81 pad 2: +20V -> GND
- C82 pad 1: GND -> /Ethernet Switch/ANALOG_3V3
- C82 pad 2: +20V -> GND
- C83 pad 1: GND -> /Ethernet Switch/ANALOG_3V3
- C83 pad 2: +20V -> GND
- C84 pad 1: GND -> /Ethernet Switch/ANALOG_3V3
- C84 pad 2: +20V -> GND
- C85 pad 1: GND -> /Ethernet Switch/ANALOG_3V3
- C85 pad 2: +20V -> GND
- C86 pad 1: GND -> /Ethernet Switch/ANALOG_3V3
- C86 pad 2: +20V -> GND
- C87 pad 1: GND -> /Ethernet Switch/ANALOG_3V3
- C87 pad 2: +20V -> GND
- C88 pad 1: /Unit 3B/BUCK_SW -> /Ethernet Switch/ANALOG_3V3
- C88 pad 2: Net-(C88-Pad2) -> GND
- C89 pad 1: /Unit 3B/M2_3V3 -> /Ethernet Switch/ANALOG_3V3
- C90 pad 1: /Unit 3B/M2_3V3 -> /Ethernet Switch/ANALOG_3V3
- C93 pad 1: /Ethernet Switch/ANALOG_3V3 -> +3V3
- C94 pad 1: /Ethernet Switch/ANALOG_3V3 -> +3V3
- C95 pad 1: /Ethernet Switch/ANALOG_3V3 -> /Ethernet Switch/ANALOG_1V1
- C96 pad 1: /Ethernet Switch/ANALOG_3V3 -> /Ethernet Switch/ANALOG_1V1
- C97 pad 1: /Ethernet Switch/ANALOG_3V3 -> +3V3
- C98 pad 1: /Ethernet Switch/ANALOG_3V3 -> +3V3
- C99 pad 1: AUX_3V3 -> /Ethernet Switch/1V1
- D1 pad 1: /Unit 1A/CM_3V3 -> Net-(D1-K)
- D1 pad 2: /Unit 1A/CM_3V3 -> /Unit 1/PCIE_PWR_EN
- D2 pad 1: /Unit 2A/CM_3V3 -> Net-(D1-K)
- D2 pad 2: /Unit 2A/CM_3V3 -> /Controller/PD12
- D3 pad 1: /Unit 3A/CM_3V3 -> Net-(D3-K)
- D3 pad 2: /Unit 3A/CM_3V3 -> /Unit 2/PCIE_PWR_EN
- D4 pad 1: /Power/PWR_MUX -> Net-(D3-K)
- D4 pad 2: /Power/VBUS -> /Controller/PD4
- D5 pad 1: /Power/PWR_MUX -> Net-(D5-K)
- D5 pad 2: CONN_VBUS -> /Unit 3/PCIE_PWR_EN
- FB1 pad 1: AUX_3V3 -> +3V3
- FB2 pad 1: AUX_1V1 -> /Ethernet Switch/1V1
- J11 pad A4: /Power/VBUS -> VBUS
- J11 pad A5: /Power/CC1 -> /USB/USB_PORT_CC1
- J11 pad A6: unconnected-(J11-D+-PadA6) -> /USB/USB_PORT_HS_D+
- J11 pad A7: unconnected-(J11-D--PadA7) -> /USB/USB_PORT_HS_D-
- J11 pad A9: /Power/VBUS -> VBUS
- J11 pad B5: /Power/CC2 -> /USB/USB_PORT_CC2
- J11 pad B6: unconnected-(J11-D+-PadB6) -> /USB/USB_PORT_HS_D+
- J11 pad B7: unconnected-(J11-D--PadB7) -> /USB/USB_PORT_HS_D-
- J2 pad 12: /Unit 1B/M2_3V3 -> /Unit 1/M2_3V3
- J2 pad 14: /Unit 1B/M2_3V3 -> /Unit 1/M2_3V3
- J2 pad 16: /Unit 1B/M2_3V3 -> /Unit 1/M2_3V3
- J2 pad 18: /Unit 1B/M2_3V3 -> /Unit 1/M2_3V3
- J2 pad 2: /Unit 1B/M2_3V3 -> /Unit 1/M2_3V3
- J2 pad 4: /Unit 1B/M2_3V3 -> /Unit 1/M2_3V3
- J2 pad 41: /Unit 1B/PCIE_RX_N -> /Unit 1/PCIE_RX+
- J2 pad 43: /Unit 1B/PCIE_RX_P -> /Unit 1/PCIE_RX-
- J2 pad 47: /Unit 1B/PCIE_TX_N -> /Unit 1/PCIE_TX+
- J2 pad 49: /Unit 1B/PCIE_TX_P -> /Unit 1/PCIE_TX-
- J2 pad 54: Net-(J2-~{PEWAKE}) -> /Unit 1/PCIE_CLK_nWAKE
- J2 pad 68: unconnected-(J2-SUSCLK-Pad68) -> /Unit 1/SUSCLK
- J2 pad 70: /Unit 1B/M2_3V3 -> /Unit 1/M2_3V3
- J2 pad 72: /Unit 1B/M2_3V3 -> /Unit 1/M2_3V3
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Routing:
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- added copper zone on B.Cu, net +20V
- added copper zone on F.Cu, net +5V
- added copper zone on In2.Cu, net /Ethernet Switch/ANALOG_1V1
- added copper zone on In3.Cu, net /Ethernet Switch/ANALOG_3V3
- added copper zone on F.Cu, net /Ethernet Switch/LX
- added copper zone on B.Cu, net /Power/BUCK_SW_3
- added copper zone on B.Cu, net /Power/BUCK_SW_5
- added copper zone on B.Cu, net /Power/PWR_MUX
- added copper zone on F.Cu, net /Power/PWR_MUX
- added copper zone on B.Cu, net /Unit 1/M2_3V3
- added copper zone on B.Cu, net /Unit 2/BUCK_SW_3
- added copper zone on B.Cu, net /Unit 2/BUCK_SW_5
- added copper zone on F.Cu, net /Unit 2/CM_5V
- added copper zone on B.Cu, net /Unit 3/BUCK_SW_3
- added copper zone on B.Cu, net /Unit 3/BUCK_SW_5
- added copper zone on F.Cu, net /Unit 3/CM_5V
- added copper zone on B.Cu, net /Unit 3/M2_3V3
- added copper zone on F.Cu, net /Unit 3/M2_3V3
- added copper zone on B.Cu, net VBUS
- added copper zone on F.Cu, net VBUS
- added copper zone on B.Cu, net VCON
- added copper zone on F.Cu, net VCON
- removed copper zone on F.Cu, net /Power/VBUS
- removed copper zone on B.Cu, net /Unit 1B/M2_3V3
- removed copper zone on B.Cu, net /Unit 2A/BUCK_SW
- removed copper zone on F.Cu, net /Unit 2A/CM_5V
- removed copper zone on B.Cu, net /Unit 2B/BUCK_SW
- removed copper zone on B.Cu, net /Unit 2B/M2_3V3
- removed copper zone on B.Cu, net /Unit 3A/BUCK_SW
- removed copper zone on F.Cu, net /Unit 3A/CM_5V
- removed copper zone on B.Cu, net /Unit 3B/BUCK_SW
- removed copper zone on B.Cu, net /Unit 3B/M2_3V3
- removed copper zone on F.Cu, net CONN_VBUS
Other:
- board size 122 x 84 mm -> 122 x 85 mm
- board text added: "Trilithon Magi v2.0"
- board text removed: "JLCJLCJLCJLC"
- board text removed: "Unit 1"
- board text removed: "Unit 1 M.2 NVMe"
- board text removed: "Unit 1 microSD"
- board text removed: "Unit 2"
- board text removed: "Unit 2 M.2 NVMe"
- board text removed: "Unit 2 microSD"
- board text removed: "Unit 3"
- board text removed: "Unit 3 M.2 NVMe"
- board text removed: "Unit 3 microSD"
